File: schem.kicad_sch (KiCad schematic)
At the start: 7 parts, among them U1 TP4056 module

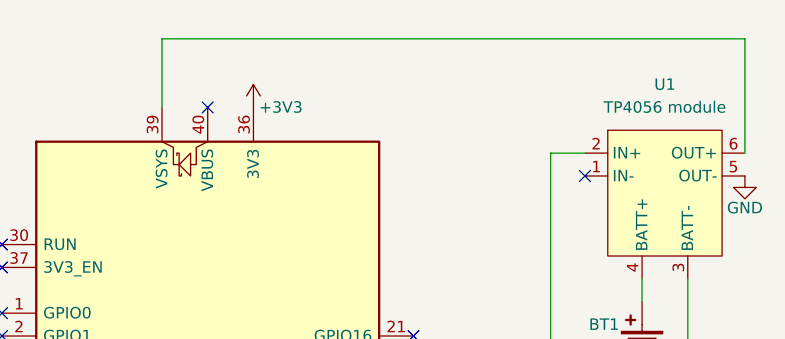
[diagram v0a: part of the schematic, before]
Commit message: Update Schematic
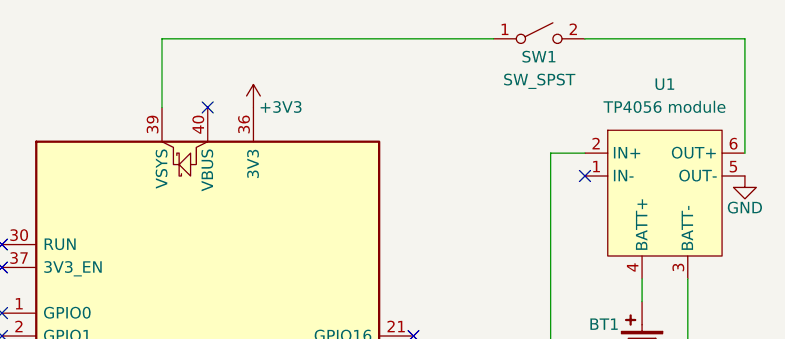
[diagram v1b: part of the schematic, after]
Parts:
- added SW1: SW_SPST, symbol Switch:SW_SPST
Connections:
- net at U1.6 (OUT+): now also SW1.2 (B); no longer A1.39 (VSYS)
- new net: A1.39 (VSYS), SW1.1 (A)
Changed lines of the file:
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@@
 	(wire
 		(pts
-			(xy 118.11 16.51) (xy 53.34 16.51)
+			(xy 118.11 16.51) (xy 100.33 16.51)
+		)
+		(stroke
+			(width 0)
+			(type default)
+		)
+	)
+	(wire
+		(pts
+			(xy 90.17 16.51) (xy 53.34 16.51)
 		)
 		(stroke
@@
 					(unit 1)
 				)
+			)
+		)
+	)
+	(symbol
+		(lib_id "Switch:SW_SPST")
+		(at 95.25 16.51 0)
+		(unit 1)
+		(body_style 1)
+		(exclude_from_sim no)
+		(in_bom yes)
+		(on_board yes)
+		(in_pos_files yes)
+		(dnp no)
+		(property "Reference" "SW1"
+			(at 95.25 18.542 0)
+			(show_name no)
+			(do_not_autoplace no)
+			(effects
+				(font
+					(size 1.27 1.27)
+				)
+			)
+		)
+		(property "Value" "SW_SPST"
+			(at 95.25 21.082 0)
+			(show_name no)
+			(do_not_autoplace no)
+			(effects
+				(font
+					(size 1.27 1.27)
+				)
+			)
+		)
+		(property "Footprint" ""
+			(at 95.25 16.51 0)
+			(hide yes)
+			(show_name no)
+			(do_not_autoplace no)
+			(effects
+				(font
+					(size 1.27 1.27)
+				)
+			)
+		)
+		(property "Datasheet" ""
+			(at 95.25 16.51 0)
+			(hide yes)
+			(show_name no)
+			(do_not_autoplace no)
+			(effects
+				(font
+					(size 1.27 1.27)
+				)
+			)
+		)
+		(property "Description" "Single Pole Single Throw (SPST) switch"
+			(at 95.25 16.51 0)
+			(hide yes)
+			(show_name no)
+			(do_not_autoplace no)
+			(effects
+				(font
+					(size 1.27 1.27)
+				)
+			)
+		)
+		(pin "1"
+		)
+		(pin "2"
+		)
+		(instances
+			(project "schem"
+				(path "/2446c2a2-99a1-4fb5-976e-2f0b9073cc8d"
+					(reference "SW1")
+					(unit 1)
+				)
